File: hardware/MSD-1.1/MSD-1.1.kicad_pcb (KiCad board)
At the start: 2 copper layers, 98.4 x 44.4 mm, 27 parts, among them J1 Conn_01x05, J2 Conn_01x03, Q1 IRF840, U1 NE555P, U2 PC817, U3 PC817

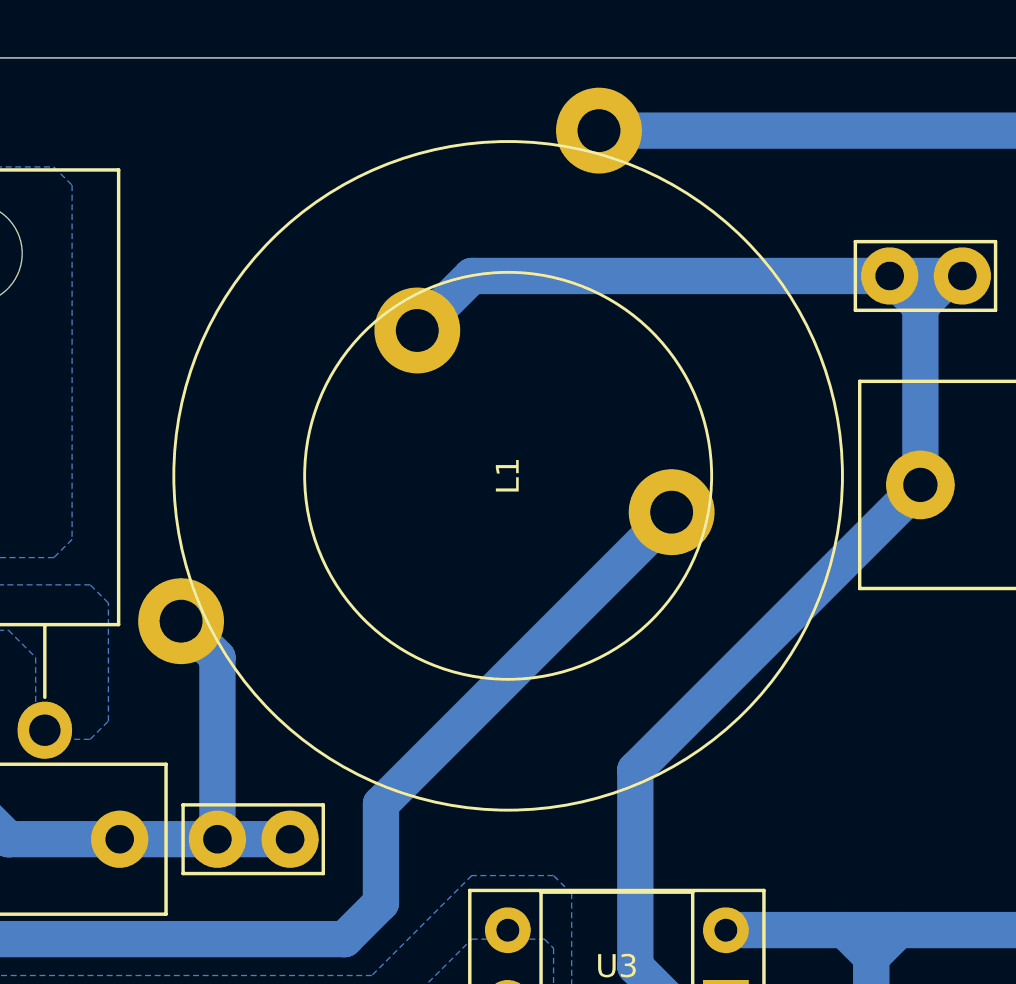
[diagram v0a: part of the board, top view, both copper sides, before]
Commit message: modified:   README.md 	deleted:    hardware/CTL-1.0/CTL-1.0-backups/CTL-1.0-2025-05-28_203806.zip 	deleted:    hardware/CTL-1.0/CTL-1.0-backups/CTL-1.0-2025-05-28_204313.zip 	deleted:    hardware/CTL-1.0/CTL-1.0-backups/CTL-1.0-2025-05-30_173028.zip 	deleted:    hardware/CTL-1.0/CTL-1.0-backups/CTL-1.0-2025-05-30_174116.zip 	deleted:    hardware/CTL-1.0/CTL-1.0-backups/CTL-1.0-2025-05-30_175122.zip 	new file:   hardware/CTL-1.0/CTL-1.0-backups/CTL-1.0-2025-07-24_151142.zip 	new file:   hardware/CTL-1.0/CTL-1.0-backups/CTL-1.0-2025-07-24_172002.zip 	new file:   hardware/CTL-1.0/CTL-1.0-backups/CTL-1.0-2025-07-25_175122.zip 	new file:   hardware/CTL-1.0/CTL-1.0-backups/CTL-1.0-2025-07-26_120011.zip 	new file:   hardware/CTL-1.0/CTL-1.0-backups/CTL-1.0-2025-07-26_120808.zip 	modified:   hardware/CTL-1.0/CTL-1.0.kicad_pcb 	modified:   hardware/CTL-1.0/CTL-1.0.kicad_pro 	new file:   hardware/CTL-1.0/CTL-1.0.step 	deleted:    hardware/MSD-1.0/MSD-1.0-backups/MSD-1.0-2025-04-11_111943.zip 	deleted:    hardware/MSD-1.0/MSD-1.0-backups/MSD-1.0-2025-04-11_113401.zip 	new file:   hardware/MSD-1.0/MSD-1.0-backups/MSD-1.0-2025-07-25_163151.zip 	new file:   hardware/MSD-1.0/MSD-1.0-backups/MSD-1.0-2025-07-25_171843.zip 	modified:   hardware/MSD-1.0/MSD-1.0.kicad_pcb 	modified:   hardware/MSD-1.0/MSD-1.0.step 	new file:   hardware/MSD-1.1/MSD-1.1-backups/MSD-1.1-2025-07-24_151252.zip 	new file:   hardware/MSD-1.1/MSD-1.1-backups/MSD-1.1-2025-07-25_152939.zip 	new file:   hardware/MSD-1.1/MSD-1.1-backups/MSD-1.1-2025-07-25_162346.zip 	new file:   hardware/MSD-1.1/MSD-1.1-backups/MSD-1.1-2025-07-25_162917.zip 	modified:   hardware/MSD-1.1/MSD-1.1.kicad_pcb 	modified:   hardware/MSD-1.1/MSD-1.1.step 	modified:   hardware/MSD-1.1/fp-info-cache 	new file:   hardware/MSD-2.0/MSD-2.0-backups/MSD-2.0-2025-07-24_151230.zip 	deleted:    hardware/PS-2.0/PS-2.0-backups/PS-2.0-2025-05-07_010425.zip 	deleted:    hardware/PS-2.0/PS-2.0-backups/PS-2.0-2025-05-09_084820.zip 	deleted:    hardware/P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
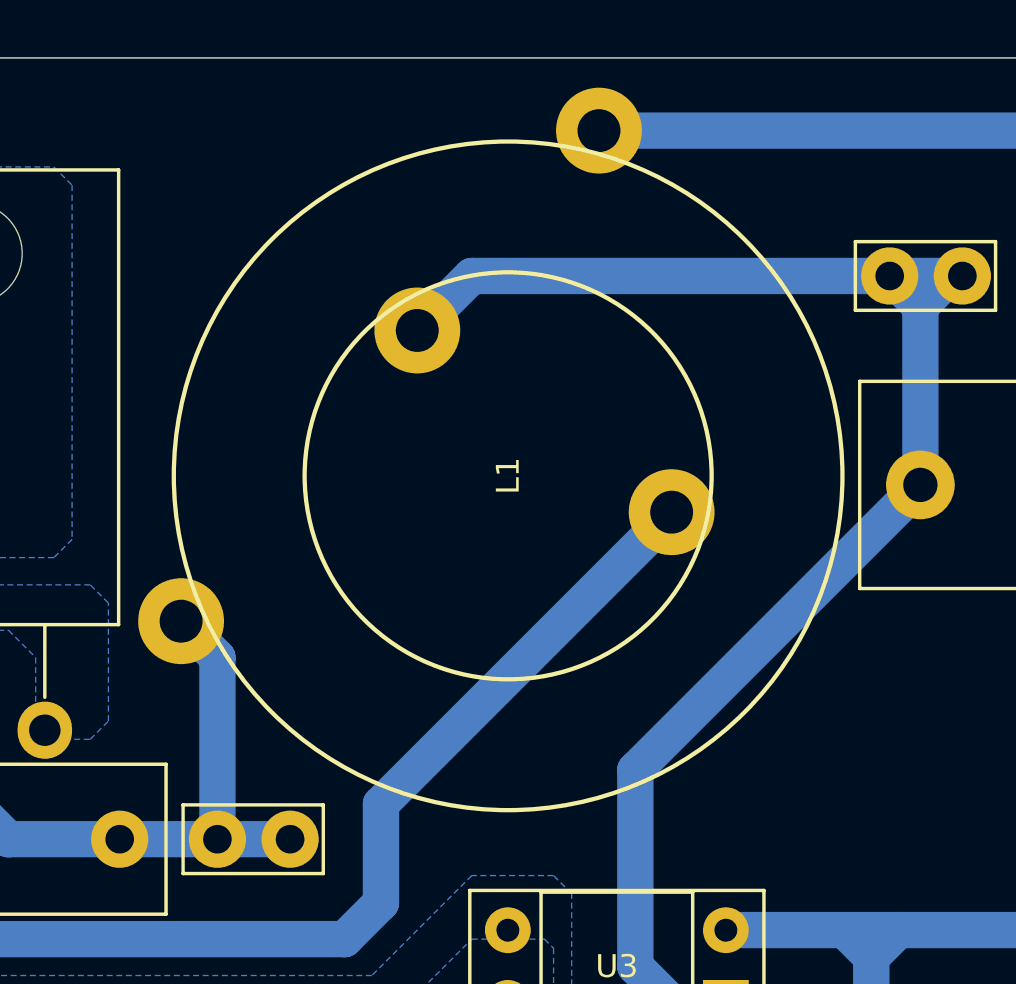
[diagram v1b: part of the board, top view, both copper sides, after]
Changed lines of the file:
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@@
 			(end 0 -11.684)
 			(stroke
-				(width 0.1)
+				(width 0.15)
 				(type default)
 			)
@@
 			(end 0 -7.112)
 			(stroke
-				(width 0.1)
+				(width 0.15)
 				(type default)
 			)
@@
 			(pintype "passive")
 		)
+		(model "/Users/margabudi/Documents/KiCad/8.0/3dmodels/Transformer/XF_Toroid_OD20_ID14_H08.stp"
+			(offset
+				(xyz 0 0 0)
+			)
+			(scale
+				(xyz 1 1 1)
+			)
+			(rotate
+				(xyz 0 0 0)
+			)
+		)
 	)
